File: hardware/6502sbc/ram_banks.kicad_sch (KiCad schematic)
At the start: 0 parts

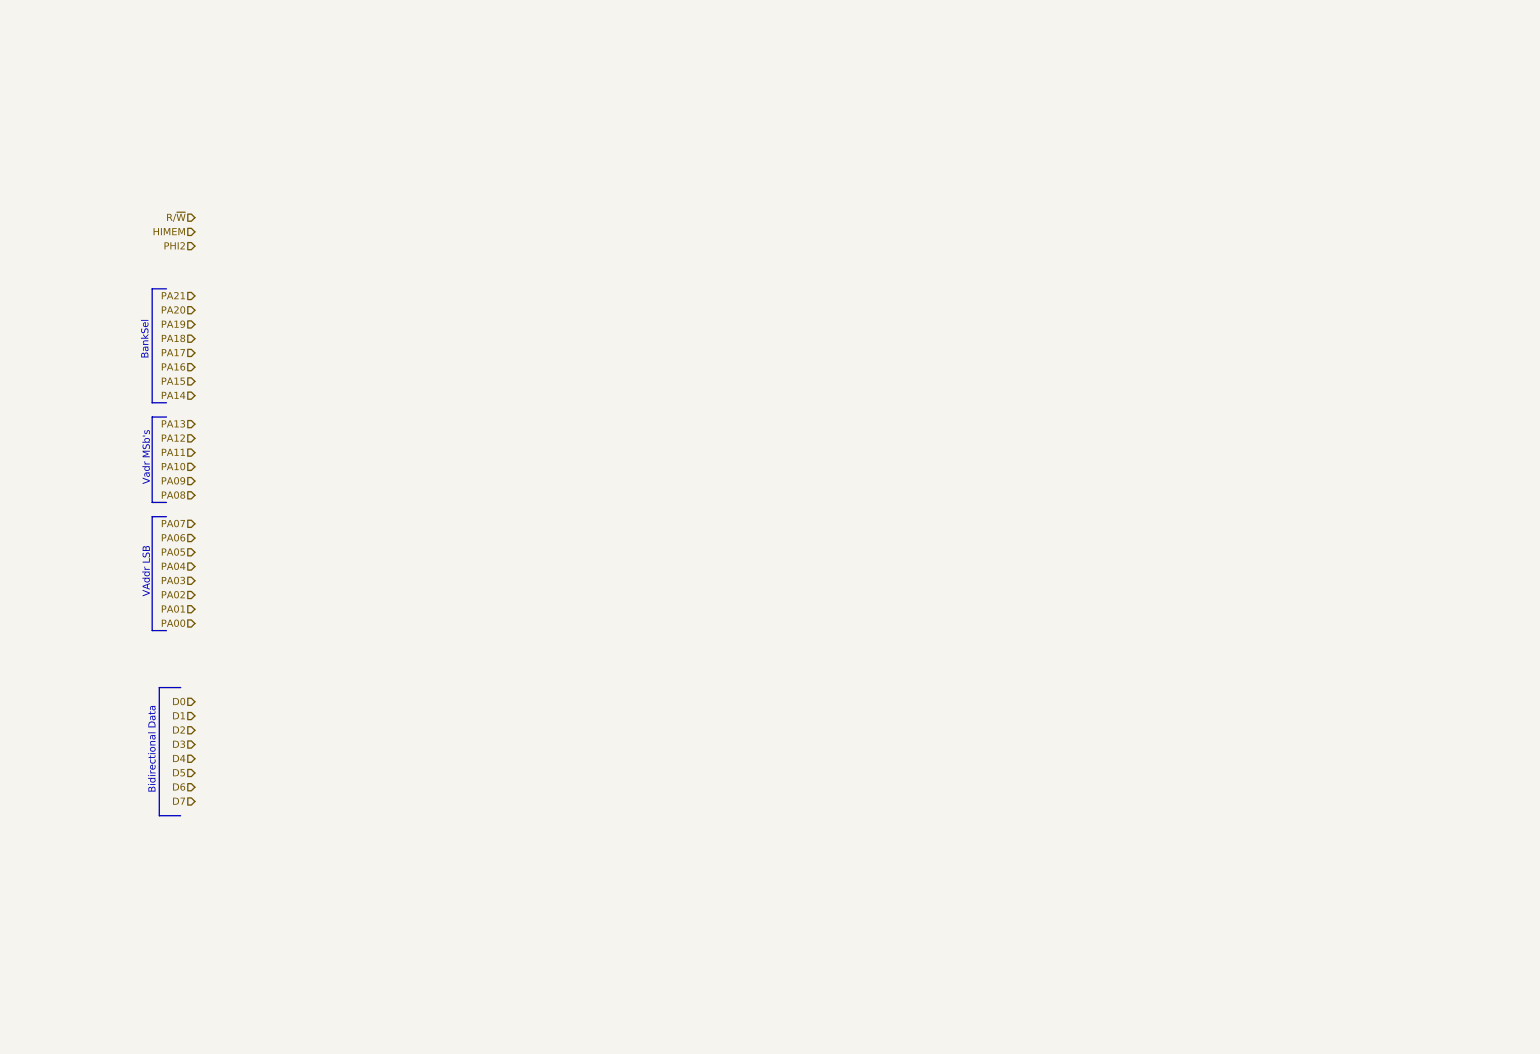
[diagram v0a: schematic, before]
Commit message: Preliminary schematic
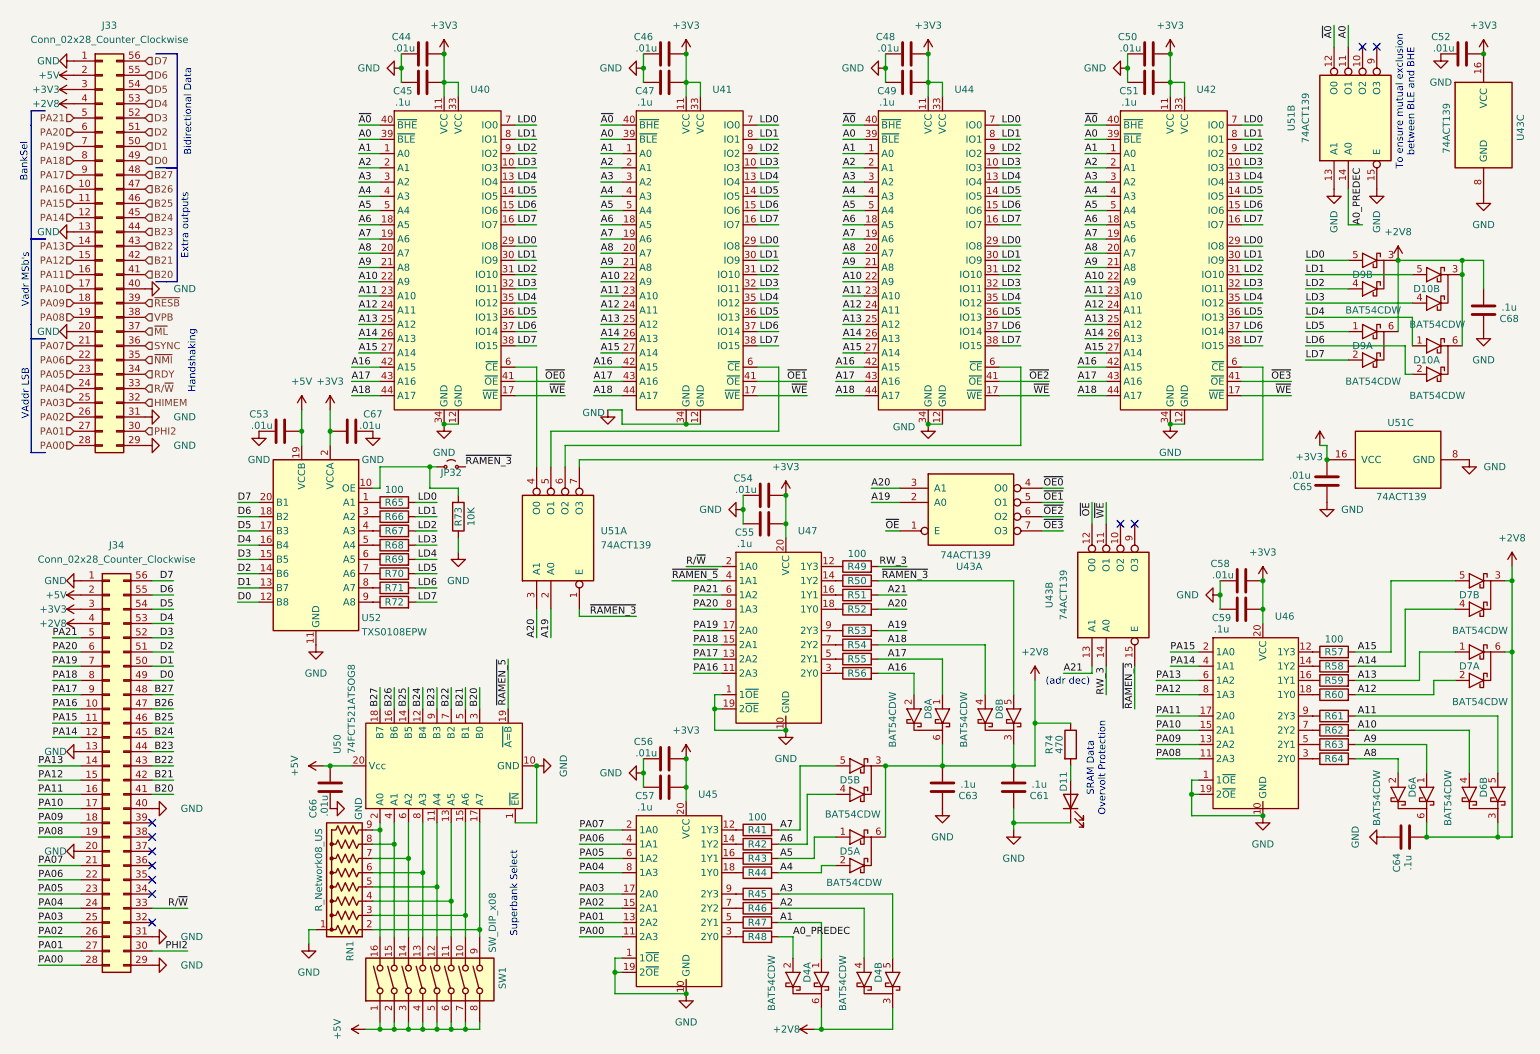
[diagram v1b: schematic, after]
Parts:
- added C44, C46, C48, C50, C52, C53, C54, C56, C58, C65, C66, C67: .01u, symbol Device:C
- added C45, C47, C49, C51, C55, C57, C59, C61, C63, C64, C68: .1u, symbol Device:C
- added D10, D4, D5, D6, D7, D8, D9: BAT54CDW, Package_TO_SOT_SMD:SOT-363_SC-70-6, symbol custom:BAT54CDW
- added D11: LED, symbol Device:LED
- added J33, J34: Conn_02x28_Counter_Clockwise, symbol Connector_Generic:Conn_02x28_Counter_Clockwise
- added JP32: Jumper_2_Small_Open, symbol Jumper:Jumper_2_Small_Open
- added R41, R42, R43, R44, R45, R46, R47, R48, R49, R50, R51, R52, R53, R54, R55, R56, R57, R58, R59, R60, R61, R62, R63, R64, R65, R66, R67, R68, R69, R70, R71, R72: 100, symbol Device:R
- added R73: 10K, symbol Device:R
- added R74: 470, symbol Device:R
- added RN1: R_Network08_US, Resistor_THT:R_Array_SIP9, symbol Device:R_Network08_US
- added SW1: SW_DIP_x08, symbol Switch:SW_DIP_x08
- added U40, U41, U42, U44: ~, Package_SO:TSOP-II-44_10.16x18.41mm_P0.8mm, symbol custom:CY7C1041DV33
- added U43, U51: 74ACT139, symbol 74xx:74LS139
- added U45, U46, U47: ~, symbol custom:74LVC244APW
- added U50: 74FCT521ATSOG8, Package_SO:SOIC-20W_7.5x12.8mm_P1.27mm, symbol custom:74FCT521AT
- added U52: TXS0108EPW, Package_SO:TSSOP-20_4.4x6.5mm_P0.65mm, symbol Logic_LevelTranslator:TXS0108EPW
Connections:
- net D0: now also J33.49 (Pin_49), J34.49 (Pin_49), U52.12 (B8)
- net D1: now also J33.50 (Pin_50), J34.50 (Pin_50), U52.13 (B7)
- net D2: now also J33.51 (Pin_51), J34.51 (Pin_51), U52.14 (B6)
- net D3: now also J33.52 (Pin_52), J34.52 (Pin_52), U52.15 (B5)
- net D4: now also J33.53 (Pin_53), J34.53 (Pin_53), U52.16 (B4)
- net D5: now also J33.54 (Pin_54), J34.54 (Pin_54), U52.17 (B3)
- net D6: now also J33.55 (Pin_55), J34.55 (Pin_55), U52.18 (B2)
- net D7: now also J33.56 (Pin_56), J34.56 (Pin_56), U52.20 (B1)
- net HIMEM: now also J33.32 (Pin_32)
- net PA00: now also J33.28 (Pin_28), J34.28 (Pin_28), U45.11 (2A3)
- net PA01: now also J33.27 (Pin_27), J34.27 (Pin_27), U45.13 (2A2)
- net PA02: now also J33.26 (Pin_26), J34.26 (Pin_26), U45.15 (2A1)
- net PA03: now also J33.25 (Pin_25), J34.25 (Pin_25), U45.17 (2A0)
- net PA04: now also J33.24 (Pin_24), J34.24 (Pin_24), U45.8 (1A3)
- net PA05: now also J33.23 (Pin_23), J34.23 (Pin_23), U45.6 (1A2)
- net PA06: now also J33.22 (Pin_22), J34.22 (Pin_22), U45.4 (1A1)
- net PA07: now also J33.21 (Pin_21), J34.21 (Pin_21), U45.2 (1A0)
- net PA08: now also J33.19 (Pin_19), J34.19 (Pin_19), U46.11 (2A3)
- net PA09: now also J33.18 (Pin_18), J34.18 (Pin_18), U46.13 (2A2)
- net PA10: now also J33.17 (Pin_17), J34.17 (Pin_17), U46.15 (2A1)
- net PA11: now also J33.16 (Pin_16), J34.16 (Pin_16), U46.17 (2A0)
- net PA12: now also J33.15 (Pin_15), J34.15 (Pin_15), U46.8 (1A3)
- net PA13: now also J33.14 (Pin_14), J34.14 (Pin_14), U46.6 (1A2)
- net PA14: now also J33.12 (Pin_12), J34.12 (Pin_12), U46.4 (1A1)
- net PA15: now also J33.11 (Pin_11), J34.11 (Pin_11), U46.2 (1A0)
- net PA16: now also J33.10 (Pin_10), J34.10 (Pin_10), U47.11 (2A3)
- net PA17: now also J33.9 (Pin_9), J34.9 (Pin_9), U47.13 (2A2)
- net PA18: now also J33.8 (Pin_8), J34.8 (Pin_8), U47.15 (2A1)
- net PA19: now also J33.7 (Pin_7), J34.7 (Pin_7), U47.17 (2A0)
- net PA20: now also J33.6 (Pin_6), J34.6 (Pin_6), U47.8 (1A3)
- net PA21: now also J33.5 (Pin_5), J34.5 (Pin_5), U47.6 (1A2)
- net PHI2: now also J33.30 (Pin_30), J34.30 (Pin_30)
- net R/~{W}: now also J33.33 (Pin_33), J34.33 (Pin_33), U47.2 (1A0)
- new net: R44.1, U45.18 (1Y0)
- new net: R42.1, U45.14 (1Y2)
- new net: R43.1, U45.16 (1Y1)
- new net: R60.1, U46.18 (1Y0)
- new net: U40.6 (~{CE}), U51.4 (O0)
- new net: U41.6 (~{CE}), U51.5 (O1)
- new net: U44.6 (~{CE}), U51.6 (O2)
- new net: U42.6 (~{CE}), U51.7 (O3)
- new net: R49.1, U47.12 (1Y3)
- new net: R50.1, U47.14 (1Y2)
- new net: R51.1, U47.16 (1Y1)
- new net: R52.1, U47.18 (1Y0)
- new net: R56.1, U47.3 (2Y0)
- new net: R55.1, U47.5 (2Y1)
- new net: R54.1, U47.7 (2Y2)
- new net: R53.1, U47.9 (2Y3)
- new net: R46.1, U45.7 (2Y2)
- new net: R65.1, U52.1 (A1)
- new net: JP32.1 (A), R73.2, U52.10 (OE)
- new net: R63.1, U46.5 (2Y1)
- new net: R41.1, U45.12 (1Y3)
- new net: R61.1, U46.9 (2Y3)
- new net: RN1.5 (R4), SW1.12, U50.11 (A4)
- new net: RN1.4 (R3), SW1.11, U50.13 (A5)
- new net: RN1.3 (R2), SW1.10, U50.15 (A6)
- new net: RN1.2 (R1), SW1.9, U50.17 (A7)
- new net: RN1.9 (R8), SW1.16, U50.2 (A0)
- new net: RN1.8 (R7), SW1.15, U50.4 (A1)
- new net: RN1.7 (R6), SW1.14, U50.6 (A2)
- new net: RN1.6 (R5), SW1.13, U50.8 (A3)
- new net: R45.1, U45.9 (2Y3)
- new net: R69.1, U52.6 (A5)
- new net: R58.1, U46.14 (1Y2)
- new net: R64.1, U46.3 (2Y0)
- new net: R48.1, U45.3 (2Y0)
- new net: R59.1, U46.16 (1Y1)
- new net: D11.2 (A), R74.2
- new net: R72.1, U52.9 (A8)
- new net: R57.1, U46.12 (1Y3)
- new net: R62.1, U46.7 (2Y2)
- new net: R47.1, U45.5 (2Y1)
- new net: R67.1, U52.4 (A3)
- new net: R70.1, U52.7 (A6)
- new net: R68.1, U52.5 (A4)
- new net: R71.1, U52.8 (A7)
- new net: R66.1, U52.3 (A2)
- new net +2V8: C61.1, C63.1, C64.1, C68.1, D10.3 (K2), D10.6 (K2), D4.3 (K2), D4.6 (K2), D5.3 (K2), D5.6 (K2), D6.3 (K2), D6.6 (K2), D7.3 (K2), D7.6 (K2), D8.3 (K2), D8.6 (K2), D9.3 (K2), D9.6 (K2), J33.4 (Pin_4), J34.4 (Pin_4), R74.1
- new net +3V3: C44.1, C45.1, C46.1, C47.1, C48.1, C49.1, C50.1, C51.1, C52.1, C54.1, C55.1, C56.1, C57.1, C58.1, C59.1, C65.1, C67.1, J33.3 (Pin_3), J34.3 (Pin_3), U40.11 (VCC), U40.33 (VCC), U41.11 (VCC), U41.33 (VCC), U42.11 (VCC), U42.33 (VCC), U43.16 (VCC), U44.11 (VCC), U44.33 (VCC), U45.20 (VCC), U46.20 (VCC), U47.20 (VCC), U51.16 (VCC), U52.2 (VCCA)
- new net +5V: C53.1, C66.1, J33.2 (Pin_2), J34.2 (Pin_2), SW1.1, SW1.2, SW1.3, SW1.4, SW1.5, SW1.6, SW1.7, SW1.8, U50.20 (Vcc), U52.19 (VCCB)
- new net A0: U40.39 (~{BLE}), U41.39 (~{BLE}), U42.39 (~{BLE}), U44.39 (~{BLE}), U51.11 (O1)
- new net A0_PREDEC: D4.2 (A02), R48.2, U51.14 (A0)
- new net A1: D4.1 (A01), R47.2, U40.1 (A0), U41.1 (A0), U42.1 (A0), U44.1 (A0)
- new net A10: D6.4 (A02), R62.2, U40.22 (A9), U41.22 (A9), U42.22 (A9), U44.22 (A9)
- new net A11: D6.5 (A12), R61.2, U40.23 (A10), U41.23 (A10), U42.23 (A10), U44.23 (A10)
- new net A12: D7.2 (A02), R60.2, U40.24 (A11), U41.24 (A11), U42.24 (A11), U44.24 (A11)
- new net A13: D7.1 (A01), R59.2, U40.25 (A12), U41.25 (A12), U42.25 (A12), U44.25 (A12)
- new net A14: D7.4 (A02), R58.2, U40.26 (A13), U41.26 (A13), U42.26 (A13), U44.26 (A13)
- new net A15: D7.5 (A12), R57.2, U40.27 (A14), U41.27 (A14), U42.27 (A14), U44.27 (A14)
- new net A16: D8.2 (A02), R56.2, U40.42 (A15), U41.42 (A15), U42.42 (A15), U44.42 (A15)
- new net A17: D8.1 (A01), R55.2, U40.43 (A16), U41.43 (A16), U42.43 (A16), U44.43 (A16)
- new net A18: D8.4 (A02), R54.2, U40.44 (A17), U41.44 (A17), U42.44 (A17), U44.44 (A17)
- new net A19: R53.2, U43.2 (A0), U51.2 (A0)
- new net A2: D4.4 (A02), R46.2, U40.2 (A1), U41.2 (A1), U42.2 (A1), U44.2 (A1)
- new net A20: R52.2, U43.3 (A1), U51.3 (A1)
- new net A21: R51.2, U43.13 (A1)
- new net A3: D4.5 (A12), R45.2, U40.3 (A2), U41.3 (A2), U42.3 (A2), U44.3 (A2)
- new net A4: D5.2 (A02), R44.2, U40.4 (A3), U41.4 (A3), U42.4 (A3), U44.4 (A3)
- new net A5: D5.1 (A01), R43.2, U40.5 (A4), U41.5 (A4), U42.5 (A4), U44.5 (A4)
- new net A6: D5.4 (A02), R42.2, U40.18 (A5), U41.18 (A5), U42.18 (A5), U44.18 (A5)
- new net A7: D5.5 (A12), R41.2, U40.19 (A6), U41.19 (A6), U42.19 (A6), U44.19 (A6)
- new net A8: D6.2 (A02), R64.2, U40.20 (A7), U41.20 (A7), U42.20 (A7), U44.20 (A7)
- new net A9: D6.1 (A01), R63.2, U40.21 (A8), U41.21 (A8), U42.21 (A8), U44.21 (A8)
- new net B20: J33.41 (Pin_41), J34.41 (Pin_41), U50.3 (B0)
- new net B21: J33.42 (Pin_42), J34.42 (Pin_42), U50.5 (B1)
- new net B22: J33.43 (Pin_43), J34.43 (Pin_43), U50.7 (B2)
- new net B23: J33.44 (Pin_44), J34.44 (Pin_44), U50.9 (B3)
- new net B24: J33.45 (Pin_45), J34.45 (Pin_45), U50.12 (B4)
- new net B25: J33.46 (Pin_46), J34.46 (Pin_46), U50.14 (B5)
- new net B26: J33.47 (Pin_47), J34.47 (Pin_47), U50.16 (B6)
- new net B27: J33.48 (Pin_48), J34.48 (Pin_48), U50.18 (B7)
- new net GND: C44.2, C45.2, C46.2, C47.2, C48.2, C49.2, C50.2, C51.2, C52.2, C53.2, C54.2, C55.2, C56.2, C57.2, C58.2, C59.2, C61.2, C63.2, C64.2, C65.2, C66.2, C67.2, C68.2, D11.1 (K), J33.1 (Pin_1), J33.13 (Pin_13), J33.20 (Pin_20), J33.29 (Pin_29), J33.31 (Pin_31), J33.40 (Pin_40), J34.1 (Pin_1), J34.13 (Pin_13), J34.20 (Pin_20), J34.29 (Pin_29), J34.31 (Pin_31), J34.40 (Pin_40), R73.1, RN1.1 (common), U40.12 (GND), U40.34 (GND), U41.12 (GND), U41.34 (GND), U42.12 (GND), U42.34 (GND), U43.8 (GND), U44.12 (GND), U44.34 (GND), U45.1 (1~{OE}), U45.10 (GND), U45.19 (2~{OE}), U46.1 (1~{OE}), U46.10 (GND), U46.19 (2~{OE}), U47.1 (1~{OE}), U47.10 (GND), U47.19 (2~{OE}), U50.1 (~{EN}), U50.10 (GND), U51.13 (A1), U51.15 (E), U51.8 (GND), U52.11 (GND)
- new net LD0: D9.5 (A12), R65.2, U40.29 (IO8), U40.7 (IO0), U41.29 (IO8), U41.7 (IO0), U42.29 (IO8), U42.7 (IO0), U44.29 (IO8), U44.7 (IO0)
- new net LD1: D10.5 (A12), R66.2, U40.30 (IO9), U40.8 (IO1), U41.30 (IO9), U41.8 (IO1), U42.30 (IO9), U42.8 (IO1), U44.30 (IO9), U44.8 (IO1)
- new net LD2: D9.4 (A02), R67.2, U40.31 (IO10), U40.9 (IO2), U41.31 (IO10), U41.9 (IO2), U42.31 (IO10), U42.9 (IO2), U44.31 (IO10), U44.9 (IO2)
- new net LD3: D10.4 (A02), R68.2, U40.10 (IO3), U40.32 (IO11), U41.10 (IO3), U41.32 (IO11), U42.10 (IO3), U42.32 (IO11), U44.10 (IO3), U44.32 (IO11)
- new net LD4: D10.1 (A01), R69.2, U40.13 (IO4), U40.35 (IO12), U41.13 (IO4), U41.35 (IO12), U42.13 (IO4), U42.35 (IO12), U44.13 (IO4), U44.35 (IO12)
- new net LD5: D9.1 (A01), R70.2, U40.14 (IO5), U40.36 (IO13), U41.14 (IO5), U41.36 (IO13), U42.14 (IO5), U42.36 (IO13), U44.14 (IO5), U44.36 (IO13)
- new net LD6: D10.2 (A02), R71.2, U40.15 (IO6), U40.37 (IO14), U41.15 (IO6), U41.37 (IO14), U42.15 (IO6), U42.37 (IO14), U44.15 (IO6), U44.37 (IO14)
- new net LD7: D9.2 (A02), R72.2, U40.16 (IO7), U40.38 (IO15), U41.16 (IO7), U41.38 (IO15), U42.16 (IO7), U42.38 (IO15), U44.16 (IO7), U44.38 (IO15)
- new net RDY: J33.34 (Pin_34)
- new net RW_3: R49.2, U43.14 (A0)
- new net SYNC: J33.36 (Pin_36)
- new net VPB: J33.38 (Pin_38)
- new net ~{A0}: U40.40 (~{BHE}), U41.40 (~{BHE}), U42.40 (~{BHE}), U44.40 (~{BHE}), U51.12 (O0)
- new net ~{ML}: J33.37 (Pin_37)
- new net ~{NMI}: J33.35 (Pin_35)
- new net ~{OE0}: U40.41 (~{OE}), U43.4 (O0)
- new net ~{OE1}: U41.41 (~{OE}), U43.5 (O1)
- new net ~{OE2}: U43.6 (O2), U44.41 (~{OE})
- new net ~{OE3}: U42.41 (~{OE}), U43.7 (O3)
- new net ~{OE}: U43.1 (E), U43.12 (O0)
- new net ~{RAMEN_3}: D8.5 (A12), JP32.2 (B), R50.2, U43.15 (E), U51.1 (E)
- new net ~{RAMEN_5}: U47.4 (1A1), U50.19 (~{A=B})
- new net ~{RESB}: J33.39 (Pin_39)
- new net ~{WE}: U40.17 (~{WE}), U41.17 (~{WE}), U42.17 (~{WE}), U43.11 (O1), U44.17 (~{WE})
- no-connect marks 0 -> 11
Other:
- note added: "(adr dec)"
- note added: "Extra outputs"
- note added: "Handshaking"
- note added: "SRAM Data Overvolt Protection"
- note added: "Superbank Select"
- note added: "To ensure mutual exclusion between BLE and BHE"
